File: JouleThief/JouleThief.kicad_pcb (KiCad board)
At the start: 2 copper layers, 44.7 x 13.2 mm, 14 parts, among them J1 Screw_Terminal_01x02, J2 Screw_Terminal_01x02, Q1 BC547, Q2 BC547

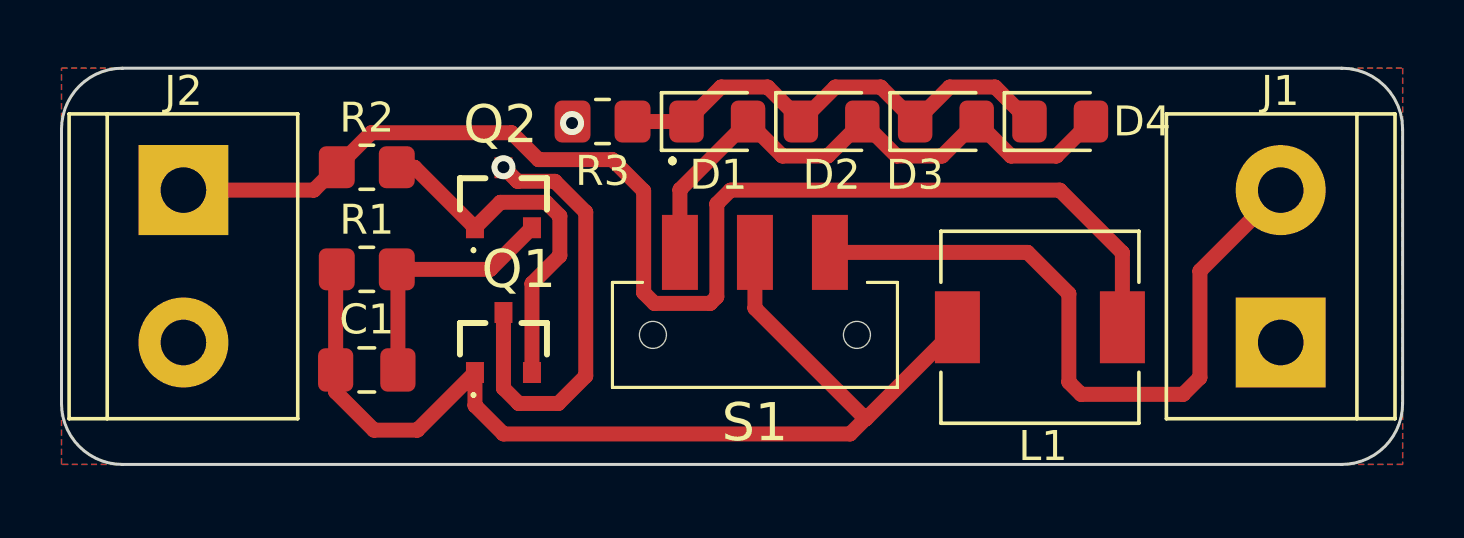
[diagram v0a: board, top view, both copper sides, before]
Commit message: production and smooth traces add
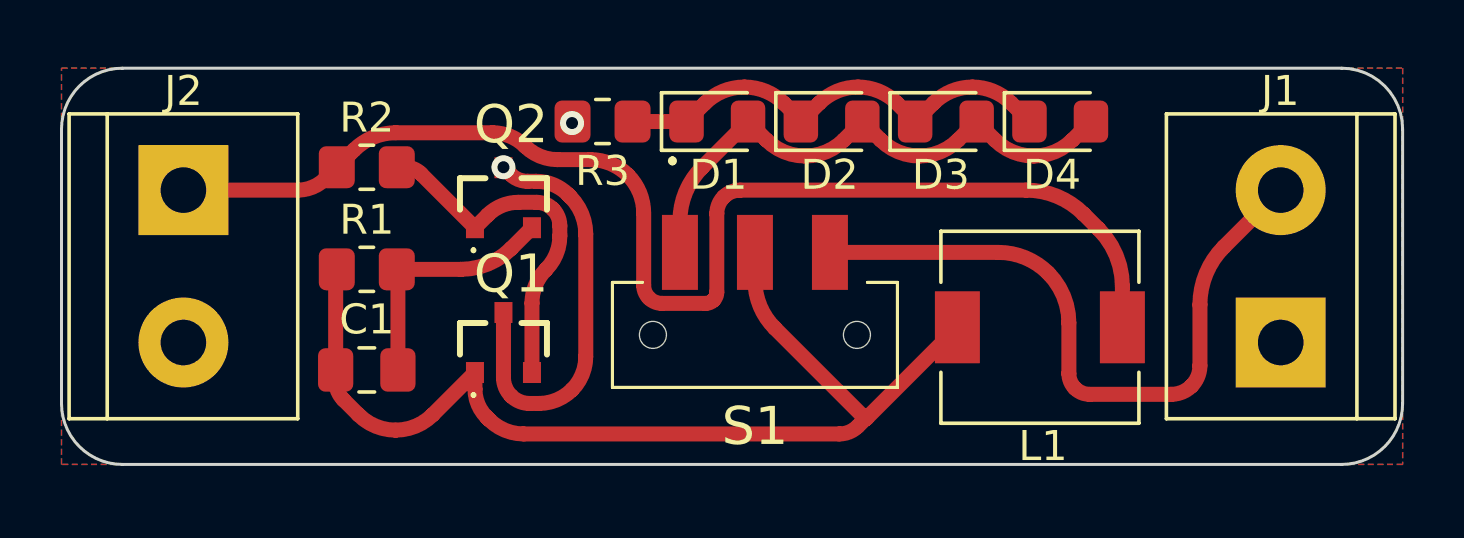
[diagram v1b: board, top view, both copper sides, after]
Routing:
- net Net-(J2-Pad1): track 43.2 -> 42.3 mm
- net Net-(D4-Pad2): track 19.6 -> 18.9 mm
- net Net-(D4-Pad1): track 16.1 -> 15.6 mm
- net Net-(J1-Pad2): track 23.6 -> 23.1 mm
